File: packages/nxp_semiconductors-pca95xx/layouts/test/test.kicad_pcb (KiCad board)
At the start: 2 copper layers, 14 parts

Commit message: Rebuild all
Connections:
- U1 pad 3: io[2]-5 -> io[2]-4
- U2 pad 1: io[0]-4 -> io[0]-5
- U2 pad 3: io[2]-4 -> io[2]-2
- U2 pad 5: io[3]-2 -> io[3]-6
- U3 pad 1: io[0]-5 -> io[0]-4
- U3 pad 2: io[1] -> io[1]-3
- U3 pad 5: io[3] -> io[3]-4
- U4 pad 10: io[7]-2 -> io[7]-1
- U4 pad 11: interrupt -> interrupt-1
- U4 pad 2: io[0]-2 -> io[0]-6
- U4 pad 3: io[1]-1 -> io[1]-5
- U4 pad 4: io[2]-3 -> io[2]-5
- U4 pad 5: io[3]-6 -> io[3]-1
- U4 pad 7: io[4] -> io[4]-2
- U4 pad 8: io[5]-3 -> io[5]-1
- U5 pad 10: io[5]-2 -> io[5]
- U5 pad 11: io[6]-3 -> io[6]-2
- U5 pad 12: io[7]-1 -> io[7]-2
- U5 pad 13: interrupt-2 -> interrupt
- U5 pad 4: io[0]-1 -> io[0]-2
- U5 pad 5: io[1]-2 -> io[1]-1
- U5 pad 6: io[2]-2 -> io[2]-3
- U5 pad 7: io[3]-4 -> io[3]-2
- U6 pad 10: io[7] -> io[7]-3
- U6 pad 11: interrupt-1 -> interrupt-3
- U6 pad 2: io[0]-6 -> io[0]-1
- U6 pad 3: io[1]-3 -> io[1]
- U6 pad 4: io[2]-6 -> io[2]
- U6 pad 5: io[3]-1 -> io[3]-5
- U6 pad 7: io[4]-2 -> io[4]
- U6 pad 8: io[5]-1 -> io[5]-2
- U7 pad 10: io[5] -> io[5]-3
- U7 pad 11: io[6]-2 -> io[6]-3
- U7 pad 12: io[7]-3 -> io[7]
- U7 pad 13: interrupt-3 -> interrupt-2
- U7 pad 5: io[1]-5 -> io[1]-2
- U7 pad 6: io[2] -> io[2]-6
- U7 pad 7: io[3]-5 -> io[3]
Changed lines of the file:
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@@
     (net 0 "")
     (net 1 "gnd")
-    (net 2 "io[1]")
-    (net 3 "io[3]")
+    (net 2 "io[1]-3")
+    (net 3 "io[3]-4")
     (net 4 "io[4]-3")
-    (net 5 "io[1]-2")
-    (net 6 "io[4]")
-    (net 7 "io[5]-2")
+    (net 5 "io[1]-1")
+    (net 6 "io[4]-2")
+    (net 7 "io[5]")
     (net 8 "io[0]")
-    (net 9 "io[7]-2")
-    (net 10 "io[3]-4")
-    (net 11 "io[7]-3")
-    (net 12 "io[3]-5")
-    (net 13 "io[2]-5")
-    (net 14 "io[6]-3")
-    (net 15 "io[3]-2")
-    (net 16 "io[6]-2")
+    (net 9 "io[7]-1")
+    (net 10 "io[3]-2")
+    (net 11 "io[7]")
+    (net 12 "io[3]")
+    (net 13 "io[2]-4")
+    (net 14 "io[6]-2")
+    (net 15 "io[3]-6")
+    (net 16 "io[6]-3")
     (net 17 "scl")
-    (net 18 "io[1]-3")
-    (net 19 "io[5]")
+    (net 18 "io[1]")
+    (net 19 "io[5]-3")
     (net 20 "io[3]-3")
-    (net 21 "io[1]-1")
+    (net 21 "io[1]-5")
     (net 22 "io[6]")
     (net 23 "io[4]-1")
     (net 24 "io[0]-3")
-    (net 25 "io[3]-6")
-    (net 26 "io[2]")
-    (net 27 "io[7]-1")
-    (net 28 "io[5]-1")
-    (net 29 "io[0]-2")
-    (net 30 "io[0]-1")
-    (net 31 "io[2]-6")
-    (net 32 "io[2]-2")
+    (net 25 "io[3]-1")
+    (net 26 "io[2]-6")
+    (net 27 "io[7]-2")
+    (net 28 "io[5]-2")
+    (net 29 "io[0]-6")
+    (net 30 "io[0]-2")
+    (net 31 "io[2]")
+    (net 32 "io[2]-3")
     (net 33 "io[1]-6")
-    (net 34 "io[3]-1")
+    (net 34 "io[3]-5")
     (net 35 "io[6]-1")
-    (net 36 "io[1]-5")
-    (net 37 "interrupt-2")
-    (net 38 "interrupt-3")
-    (net 39 "io[4]-2")
-    (net 40 "io[2]-4")
+    (net 36 "io[1]-2")
+    (net 37 "interrupt")
+    (net 38 "interrupt-2")
+    (net 39 "io[4]")
+    (net 40 "io[2]-2")
     (net 41 "sda")
-    (net 42 "io[7]")
-    (net 43 "io[0]-4")
+    (net 42 "io[7]-3")
+    (net 43 "io[0]-5")
     (net 44 "io[1]-4")
-    (net 45 "interrupt")
-    (net 46 "io[5]-3")
-    (net 47 "io[2]-3")
-    (net 48 "io[0]-5")
-    (net 49 "io[0]-6")
+    (net 45 "interrupt-1")
+    (net 46 "io[5]-1")
+    (net 47 "io[2]-5")
+    (net 48 "io[0]-4")
+    (net 49 "io[0]-1")
     (net 50 "io[2]-1")
-    (net 51 "interrupt-1")
+    (net 51 "interrupt-3")
     (net 52 "vdd")
     (footprint "atopile:TSSOP-16_L5.0-W4.4-P0.65-LS6.4-BL-4f6acc"
@@
             (size 0.34 1.73)
             (layers "F.Cu" "F.Mask" "F.Paste")
-            (net 36 "io[1]-5")
+            (net 36 "io[1]-2")
         )
         (pad "6" smd oval
@@
             (size 0.34 1.73)
             (layers "F.Cu" "F.Mask" "F.Paste")
-            (net 26 "io[2]")
+            (net 26 "io[2]-6")
         )
         (pad "7" smd oval
@@
             (size 0.34 1.73)
             (layers "F.Cu" "F.Mask" "F.Paste")
-            (net 12 "io[3]-5")
+            (net 12 "io[3]")
         )
         (pad "8" smd oval
@@
             (size 0.34 1.73)
             (layers "F.Cu" "F.Mask" "F.Paste")
-            (net 19 "io[5]")
+            (net 19 "io[5]-3")
         )
         (pad "11" smd oval
@@
             (size 0.34 1.73)
             (layers "F.Cu" "F.Mask" "F.Paste")
-            (net 16 "io[6]-2")
+            (net 16 "io[6]-3")
         )
         (pad "12" smd oval
@@
             (size 0.34 1.73)
             (layers "F.Cu" "F.Mask" "F.Paste")
-            (net 11 "io[7]-3")
+            (net 11 "io[7]")
         )
         (pad "13" smd oval
@@
             (size 0.34 1.73)
             (layers "F.Cu" "F.Mask" "F.Paste")
-            (net 38 "interrupt-3")
+            (net 38 "interrupt-2")
         )
         (pad "14" smd oval
@@
             (size 0.3 0.85)
             (layers "F.Cu" "F.Mask" "F.Paste")
-            (net 13 "io[2]-5")
+            (net 13 "io[2]-4")
         )
         (pad "4" smd oval
@@
             (size 0.37 1.35)
             (layers "F.Cu" "F.Mask" "F.Paste")
-            (net 48 "io[0]-5")
+            (net 48 "io[0]-4")
         )
         (pad "2" smd oval
@@
             (size 0.37 1.35)
             (layers "F.Cu" "F.Mask" "F.Paste")
-            (net 2 "io[1]")
+            (net 2 "io[1]-3")
         )
         (pad "3" smd oval
@@
             (size 0.37 1.35)
             (layers "F.Cu" "F.Mask" "F.Paste")
-            (net 3 "io[3]")
+            (net 3 "io[3]-4")
         )
         (pad "6" smd oval
@@
             (size 0.35 1)
             (layers "F.Cu" "F.Mask" "F.Paste")
-            (net 49 "io[0]-6")
+            (net 49 "io[0]-1")
         )
         (pad "3" smd rect
@@
             (size 0.35 1)
             (layers "F.Cu" "F.Mask" "F.Paste")
-            (net 18 "io[1]-3")
+            (net 18 "io[1]")
         )
         (pad "4" smd rect
@@
             (size 0.35 1)
             (layers "F.Cu" "F.Mask" "F.Paste")
-            (net 31 "io[2]-6")
+            (net 31 "io[2]")
         )
         (pad "5" smd rect
@@
             (size 0.35 1)
             (layers "F.Cu" "F.Mask" "F.Paste")
-            (net 34 "io[3]-1")
+            (net 34 "io[3]-5")
         )
         (pad "6" smd rect
@@
             (size 0.35 1)
             (layers "F.Cu" "F.Mask" "F.Paste")
-            (net 39 "io[4]-2")
+            (net 39 "io[4]")
         )
         (pad "8" smd rect
@@
             (size 0.35 1)
             (layers "F.Cu" "F.Mask" "F.Paste")
-            (net 28 "io[5]-1")
+            (net 28 "io[5]-2")
         )
         (pad "9" smd rect
@@
             (size 0.35 1)
             (layers "F.Cu" "F.Mask" "F.Paste")
-            (net 42 "io[7]")
+            (net 42 "io[7]-3")
         )
         (pad "11" smd rect
@@
             (size 0.35 1)
             (layers "F.Cu" "F.Mask" "F.Paste")
-            (net 51 "interrupt-1")
+            (net 51 "interrupt-3")
         )
         (pad "12" smd rect
@@
             (size 0.6 1.8)
             (layers "F.Cu" "F.Mask" "F.Paste")
-            (net 43 "io[0]-4")
+            (net 43 "io[0]-5")
         )
         (pad "2" smd rect
@@
             (size 0.6 1.8)
             (layers "F.Cu" "F.Mask" "F.Paste")
-            (net 40 "io[2]-4")
+            (net 40 "io[2]-2")
         )
         (pad "4" smd rect
@@
             (size 0.6 1.8)
             (layers "F.Cu" "F.Mask" "F.Paste")
-            (net 15 "io[3]-2")
+            (net 15 "io[3]-6")
         )
         (pad "6" smd rect
@@
             (size 0.34 1.73)
             (layers "F.Cu" "F.Mask" "F.Paste")
-            (net 30 "io[0]-1")
+            (net 30 "io[0]-2")
         )
         (pad "5" smd oval
@@
             (size 0.34 1.73)
             (layers "F.Cu" "F.Mask" "F.Paste")
-            (net 5 "io[1]-2")
+            (net 5 "io[1]-1")
         )
         (pad "6" smd oval
@@
             (size 0.34 1.73)
             (layers "F.Cu" "F.Mask" "F.Paste")
-            (net 32 "io[2]-2")
+            (net 32 "io[2]-3")
         )
         (pad "7" smd oval
@@
             (size 0.34 1.73)
             (layers "F.Cu" "F.Mask" "F.Paste")
-            (net 10 "io[3]-4")
+            (net 10 "io[3]-2")
         )
         (pad "8" smd oval
@@
             (size 0.34 1.73)
             (layers "F.Cu" "F.Mask" "F.Paste")
-            (net 7 "io[5]-2")
+            (net 7 "io[5]")
         )
         (pad "11" smd oval
@@
             (size 0.34 1.73)
             (layers "F.Cu" "F.Mask" "F.Paste")
-            (net 14 "io[6]-3")
+            (net 14 "io[6]-2")
         )
         (pad "12" smd oval
@@
             (size 0.34 1.73)
             (layers "F.Cu" "F.Mask" "F.Paste")
-            (net 27 "io[7]-1")
+            (net 27 "io[7]-2")
         )
         (pad "13" smd oval
@@
             (size 0.34 1.73)
             (layers "F.Cu" "F.Mask" "F.Paste")
-            (net 37 "interrupt-2")
+            (net 37 "interrupt")
         )
         (pad "14" smd oval
@@
             (size 0.35 1)
             (layers "F.Cu" "F.Mask" "F.Paste")
-            (net 29 "io[0]-2")
+            (net 29 "io[0]-6")
         )
         (pad "3" smd rect
@@
             (size 0.35 1)
             (layers "F.Cu" "F.Mask" "F.Paste")
-            (net 21 "io[1]-1")
+            (net 21 "io[1]-5")
         )
         (pad "4" smd rect
@@
             (size 0.35 1)
             (layers "F.Cu" "F.Mask" "F.Paste")
-            (net 47 "io[2]-3")
+            (net 47 "io[2]-5")
         )
         (pad "5" smd rect
@@
             (size 0.35 1)
             (layers "F.Cu" "F.Mask" "F.Paste")
-            (net 25 "io[3]-6")
+            (net 25 "io[3]-1")
         )
         (pad "6" smd rect
@@
             (size 0.35 1)
             (layers "F.Cu" "F.Mask" "F.Paste")
-            (net 6 "io[4]")
+            (net 6 "io[4]-2")
         )
         (pad "8" smd rect
@@
             (size 0.35 1)
             (layers "F.Cu" "F.Mask" "F.Paste")
-            (net 46 "io[5]-3")
+            (net 46 "io[5]-1")
         )
         (pad "9" smd rect
@@
             (size 0.35 1)
             (layers "F.Cu" "F.Mask" "F.Paste")
-            (net 9 "io[7]-2")
+            (net 9 "io[7]-1")
         )
         (pad "11" smd rect
@@
             (size 0.35 1)
             (layers "F.Cu" "F.Mask" "F.Paste")
-            (net 45 "interrupt")
+            (net 45 "interrupt-1")
         )
         (pad "12" smd rect

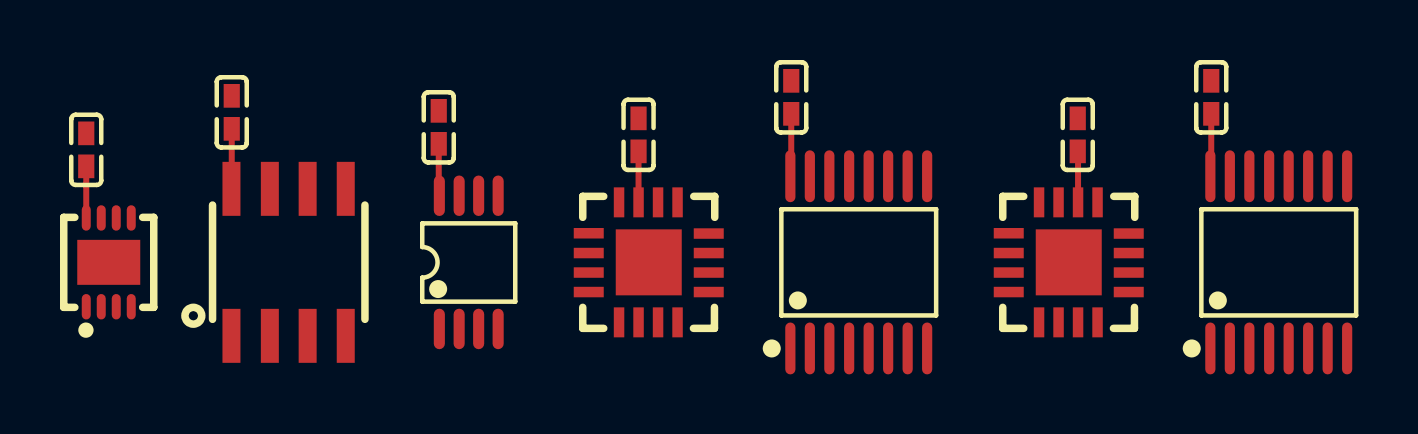
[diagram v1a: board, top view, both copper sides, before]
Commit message: WIP update pca95xx
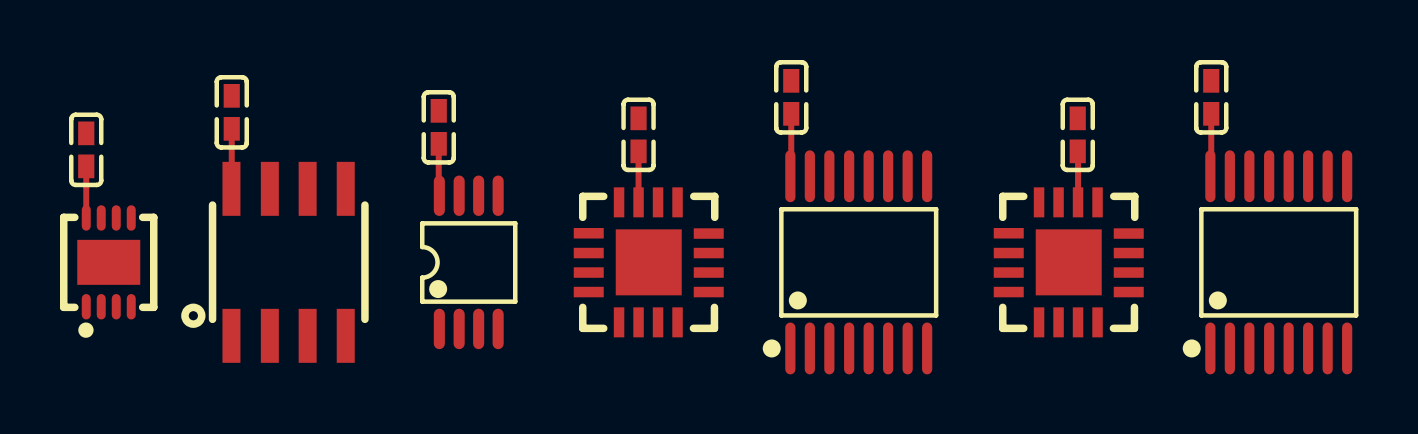
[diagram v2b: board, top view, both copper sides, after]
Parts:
- C1, C2, C3, C4, C5, C6, C7: footprint atopile:C0402-b3ef17 -> Samsung_Electro_Mechanics_CL05B104KO5NNNC:C0402
- U1: footprint atopile:HVSON-8_L3.0-W3.0-P0.50-BL-EP-57c643 -> NXP_Semicon_PCA9536TK_118:HVSON-8_L3.0-W3.0-P0.50-BL-EP
- U2: footprint atopile:SO-8_L4.9-W3.9-P1.27-LS6.0-BL-277a6b -> NXP_Semicon_PCA9536D_118:SO-8_L4.9-W3.9-P1.27-LS6.0-BL
- U3: footprint atopile:TSSOP-8_L3.0-W3.0-P0.65-LS4.9-BL-95fce5 -> NXP_Semicon_PCA9536DP_118:TSSOP-8_L3.0-W3.0-P0.65-LS4.9-BL
- U4: footprint atopile:HVQFN-16_L4.0-W4.0-P0.65-TL-EP2.2-8bbd7b -> NXP_Semicon_PCA9554BS_118:HVQFN-16_L4.0-W4.0-P0.65-TL-EP2.2
- U5: footprint atopile:TSSOP-16_L5.0-W4.4-P0.65-LS6.4-BL-4f6acc -> NXP_Semicon_PCA9554PW_118:TSSOP-16_L5.0-W4.4-P0.65-LS6.4-BL
- U6: footprint atopile:HVQFN-16_L4.0-W4.0-P0.65-TL-EP2.2-8bbd7b -> NXP_Semicon_PCA9554ABS_118:HVQFN-16_L4.0-W4.0-P0.65-TL-EP2.2
- U7: footprint atopile:TSSOP-16_L5.0-W4.4-P0.65-LS6.4-BL-4f6acc -> NXP_Semicon_PCA9554APW_118:TSSOP-16_L5.0-W4.4-P0.65-LS6.4-BL
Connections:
- U1 pad 1: io[0]-3 -> io[0]-4
- U1 pad 2: io[1]-4 -> io[1]-6
- U1 pad 3: io[2]-4 -> io[2]
- U1 pad 5: io[3]-3 -> io[3]
- U2 pad 1: io[0]-5 -> io[0]-1
- U2 pad 2: io[1]-6 -> io[1]-5
- U2 pad 5: io[3]-6 -> io[3]-1
- U3 pad 1: io[0]-4 -> io[0]-2
- U3 pad 3: io[2]-1 -> io[2]-5
- U3 pad 5: io[3]-4 -> io[3]-3
- U4 pad 10: io[7]-1 -> io[7]
- U4 pad 11: interrupt-1 -> interrupt
- U4 pad 2: io[0]-6 -> io[0]
- U4 pad 3: io[1]-5 -> io[1]
- U4 pad 4: io[2]-5 -> io[2]-1
- U4 pad 5: io[3]-1 -> io[3]-2
- U4 pad 8: io[5]-1 -> io[5]-3
- U5 pad 10: io[5] -> io[5]-2
- U5 pad 11: io[6]-2 -> io[6]-3
- U5 pad 13: interrupt -> interrupt-1
- U5 pad 4: io[0]-2 -> io[0]-6
- U5 pad 5: io[1]-1 -> io[1]-2
- U5 pad 6: io[2]-3 -> io[2]-6
- U5 pad 7: io[3]-2 -> io[3]-4
- U6 pad 10: io[7]-3 -> io[7]-1
- U6 pad 2: io[0]-1 -> io[0]-3
- U6 pad 3: io[1] -> io[1]-4
- U6 pad 4: io[2] -> io[2]-3
- U6 pad 8: io[5]-2 -> io[5]
- U7 pad 10: io[5]-3 -> io[5]-1
- U7 pad 11: io[6]-3 -> io[6]-2
- U7 pad 12: io[7] -> io[7]-3
- U7 pad 4: io[0] -> io[0]-5
- U7 pad 5: io[1]-2 -> io[1]-1
- U7 pad 6: io[2]-6 -> io[2]-4
- U7 pad 7: io[3] -> io[3]-6
